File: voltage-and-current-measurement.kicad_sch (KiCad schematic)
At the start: 76 parts

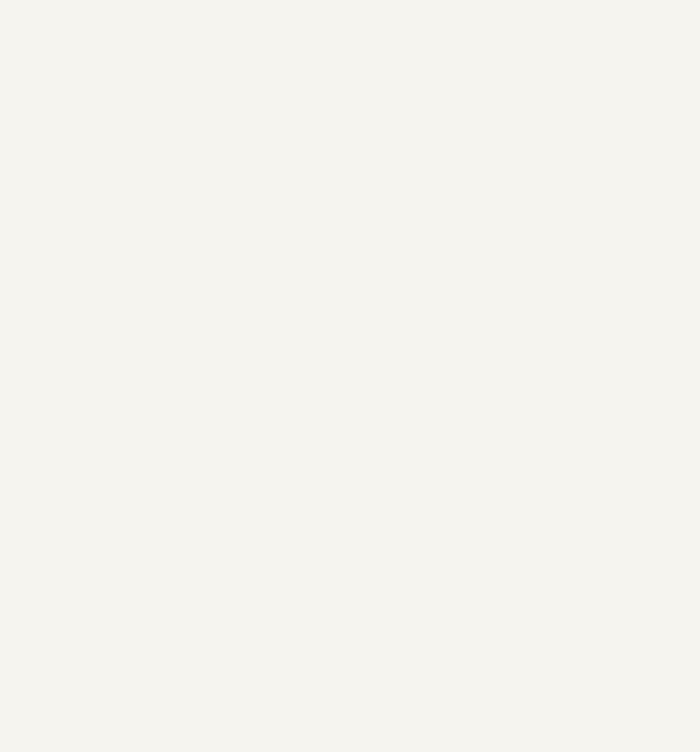
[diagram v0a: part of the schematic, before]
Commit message: WIP Sch components standarization
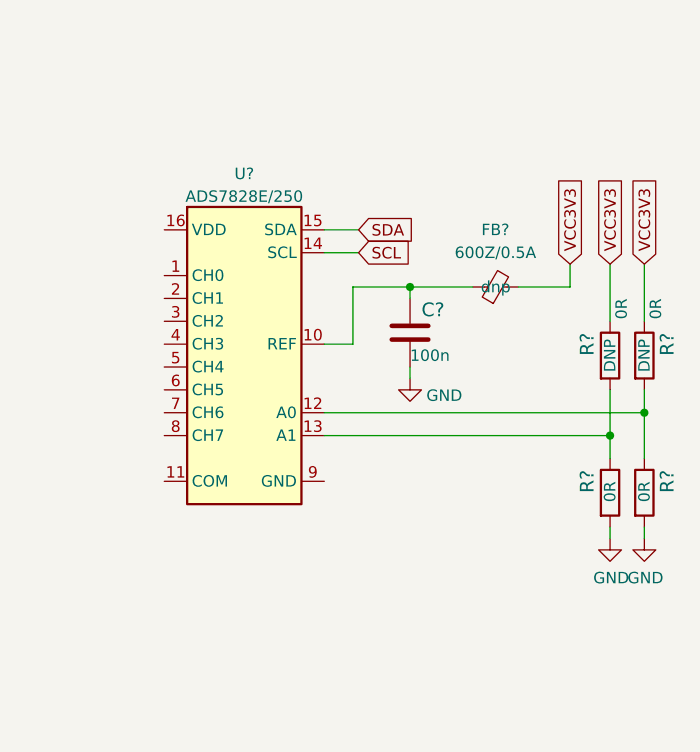
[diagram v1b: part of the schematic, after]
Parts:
- added C?: C_100n_0402, antmicro-footprints:C_0402_1005Metric, symbol antmicroCapacitors0402:C_100n_0402
- added FB?: FB_600Z_0.5A_Murata-BLM18AG_0603, antmicro-footprints:FB_0603_1608Metric, symbol antmicroFerriteBeadsandChips:FB_600Z_0.5A_Murata-BLM18AG_0603
- added R? (x4): R_0R_0402, antmicro-footprints:R_0402_1005Metric, symbol antmicroResistors0402:R_0R_0402
- added U?: ADS7828, antmicro-footprints:TSSOP-16_4.4x5mm_P0.65mm, symbol antmicroDataAcquisitionAnalogtoDigitalConvertersADC:ADS7828
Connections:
- net GND: now also C?.2, R?.2, R?.2
- net SCL: now also U?.14 (SCL)
- net SDA: now also U?.15 (SDA)
- net VCC3V3: now also FB?.2, R?.1, R?.1
- new net: R?.1, R?.2, U?.12 (A0)
- new net: R?.1, R?.2, U?.13 (A1)
- new net: C?.1, FB?.1, U?.10 (REF)

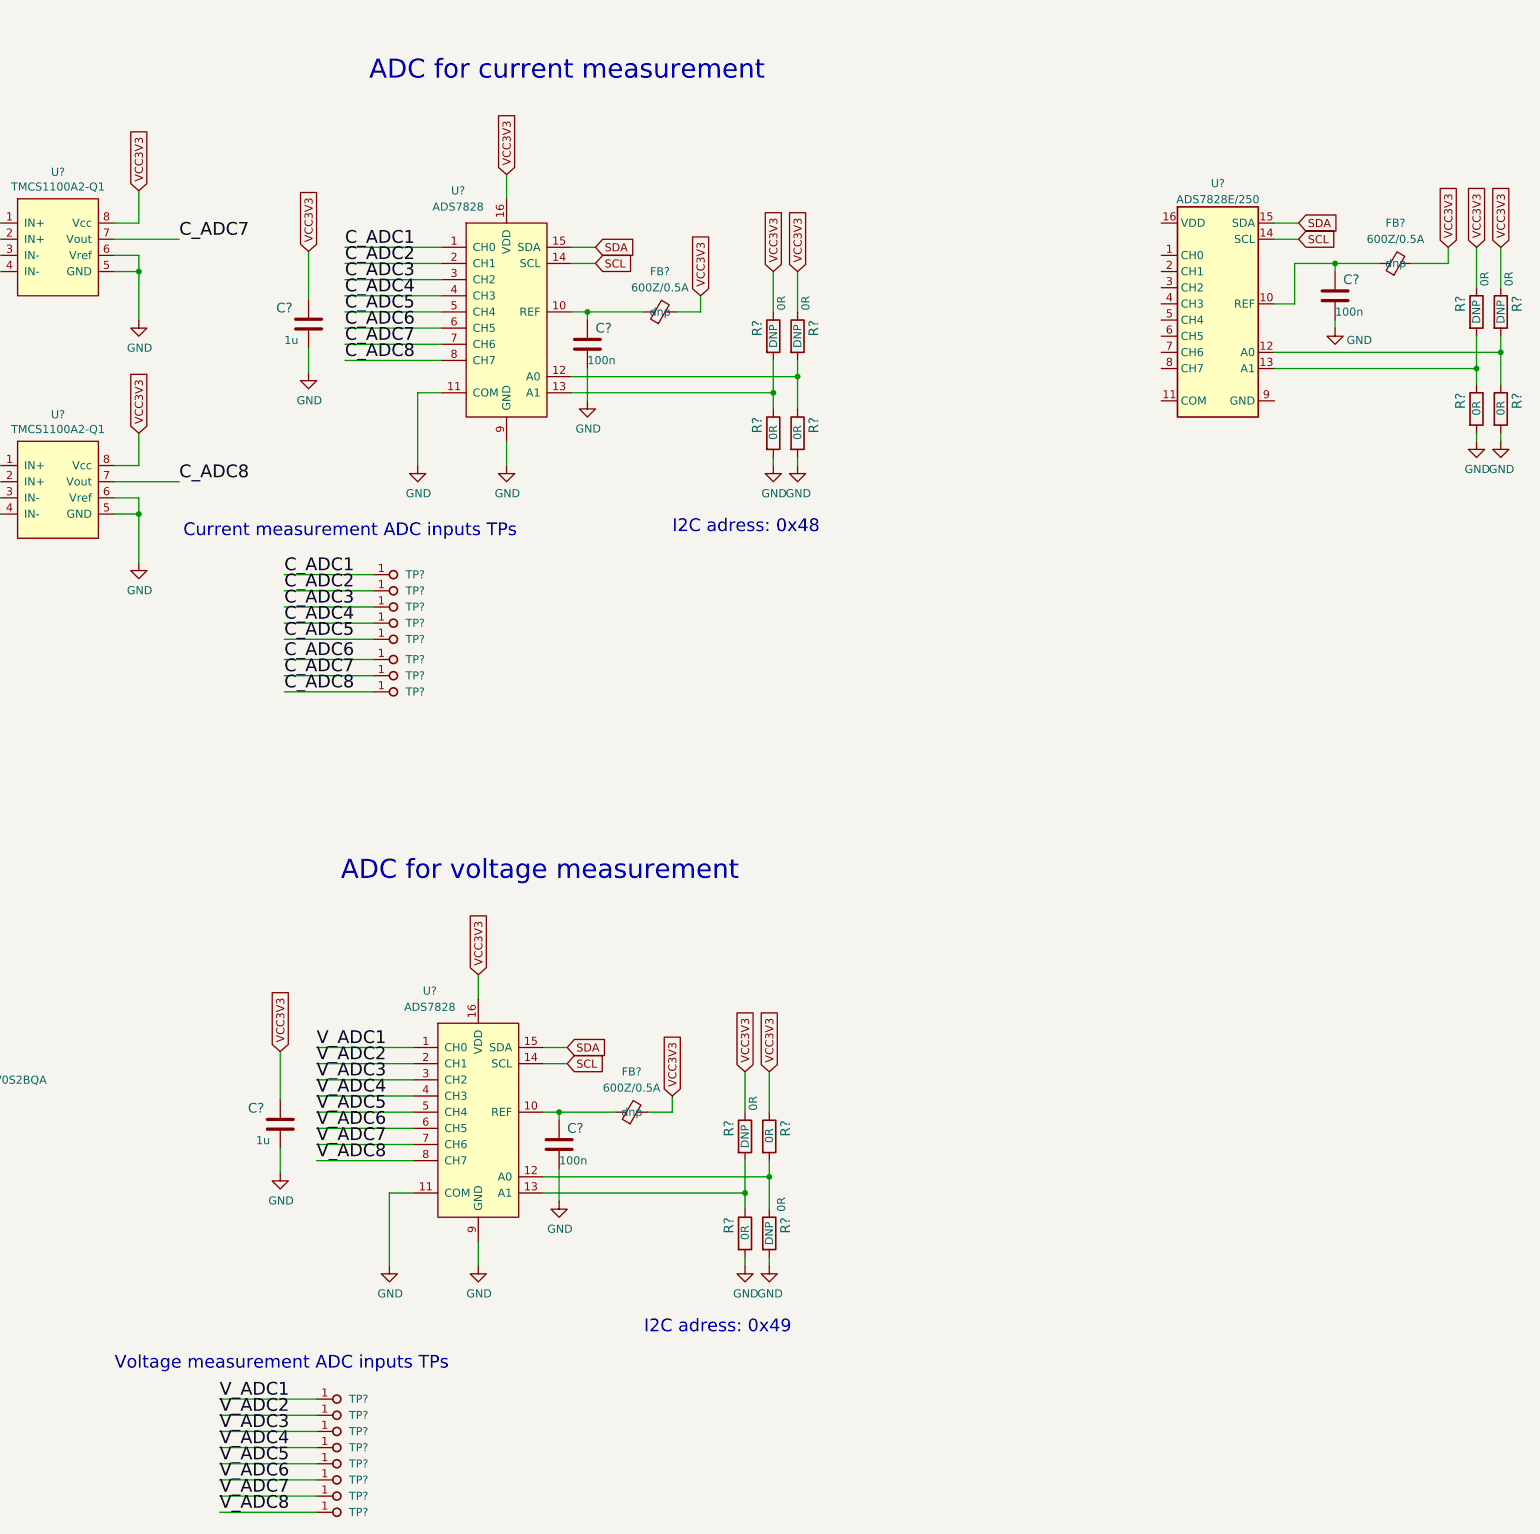
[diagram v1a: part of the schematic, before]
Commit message: WIP Standarization
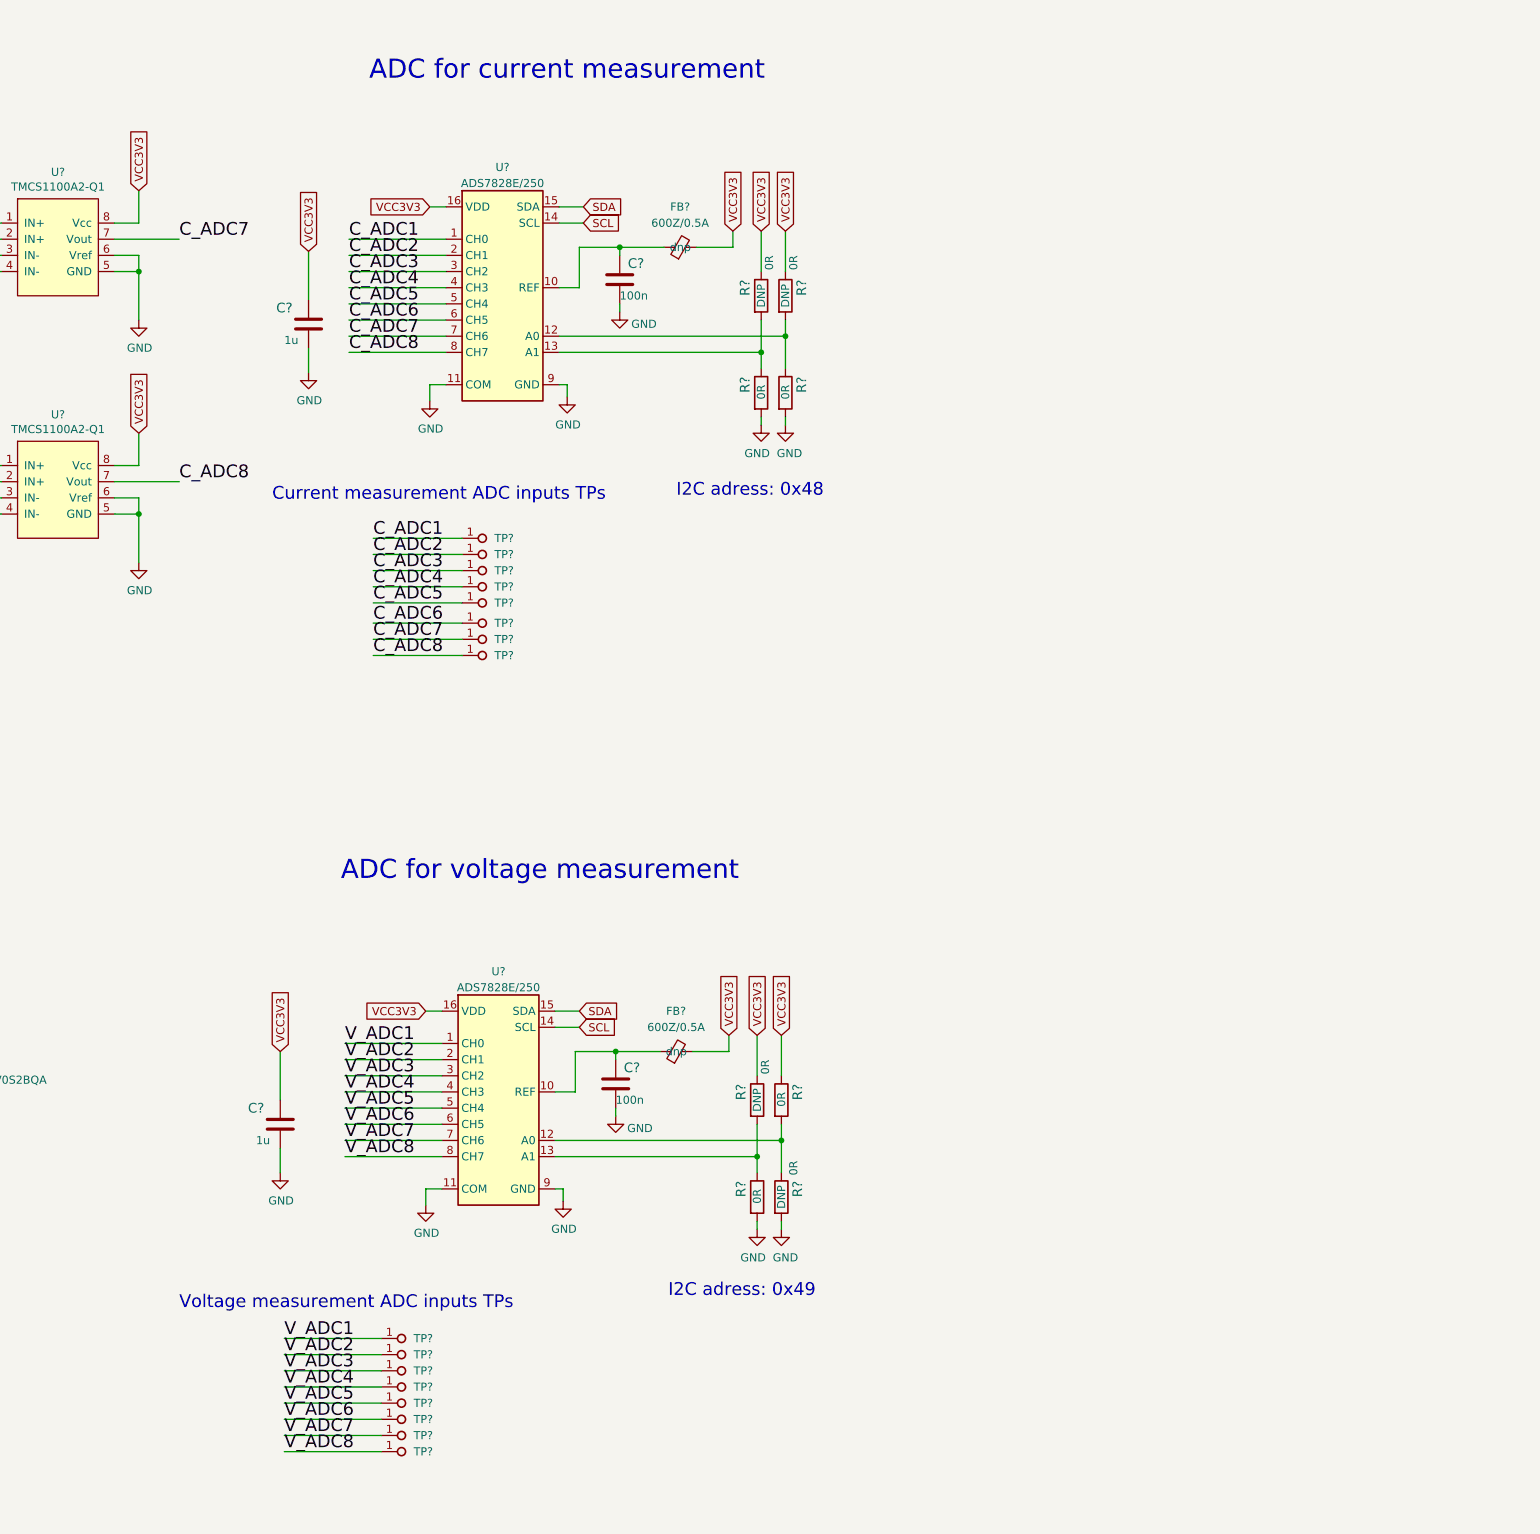
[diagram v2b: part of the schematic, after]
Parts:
- removed C? (x2): C_100n_0402, antmicro-footprints:C_0402_1005Metric, symbol antmicroCapacitors0402:C_100n_0402
- removed FB? (x2): FB_600Z_0.5A_Murata-BLM18AG_0603, antmicro-footprints:FB_0603_1608Metric, symbol antmicroFerriteBeadsandChips:FB_600Z_0.5A_Murata-BLM18AG_0603
- removed R? (x8): R_0R_0402, antmicro-footprints:R_0402_1005Metric, symbol antmicroResistors0402:R_0R_0402
- removed U? (x2): ADS7828, gpu-cluster-backplane-footprints:TSSOP-16_4.4x5mm_P0.65mm, symbol gpu-cluster-backplane:ADS7828
- added C?: C_100n_0402, antmicro-footprints:C_0402_1005Metric, symbol antmicroCapacitors0402:C_100n_0402
- added FB?: FB_600Z_0.5A_Murata-BLM18AG_0603, antmicro-footprints:FB_0603_1608Metric, symbol antmicroFerriteBeadsandChips:FB_600Z_0.5A_Murata-BLM18AG_0603
- added R? (x4): R_0R_0402, antmicro-footprints:R_0402_1005Metric, symbol antmicroResistors0402:R_0R_0402
- added U?: ADS7828, antmicro-footprints:TSSOP-16_4.4x5mm_P0.65mm, symbol antmicroDataAcquisitionAnalogtoDigitalConvertersADC:ADS7828
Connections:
- net C_ADC1: now also U?.1 (CH0)
- net C_ADC2: now also U?.2 (CH1)
- net C_ADC3: now also U?.3 (CH2)
- net C_ADC4: now also U?.4 (CH3)
- net C_ADC5: now also U?.5 (CH4)
- net C_ADC6: now also U?.6 (CH5)
- net C_ADC7: now also U?.7 (CH6)
- net C_ADC8: now also U?.8 (CH7)
- net GND: now also U?.11 (COM), U?.9 (GND), C?.2, R?.2, R?.2, U?.11 (COM), U?.9 (GND)
- net SCL: now also U?.14 (SCL)
- net SDA: now also U?.15 (SDA)
- net VCC3V3: now also U?.16 (VDD), FB?.2, R?.1, R?.1, U?.16 (VDD)
- net V_ADC1: now also U?.1 (CH0)
- net V_ADC2: now also U?.2 (CH1)
- net V_ADC3: now also U?.3 (CH2)
- net V_ADC4: now also U?.4 (CH3)
- net V_ADC5: now also U?.5 (CH4)
- net V_ADC6: now also U?.6 (CH5)
- net V_ADC7: now also U?.7 (CH6)
- net V_ADC8: now also U?.8 (CH7)
- new net: R?.1, R?.2, U?.12 (A0)
- new net: R?.1, R?.2, U?.13 (A1)
- new net: C?.1, FB?.1, U?.10 (REF)
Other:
- moved on the sheet: C?, FB?, R?, TP?, U?
